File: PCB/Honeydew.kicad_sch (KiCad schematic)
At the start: 9 parts

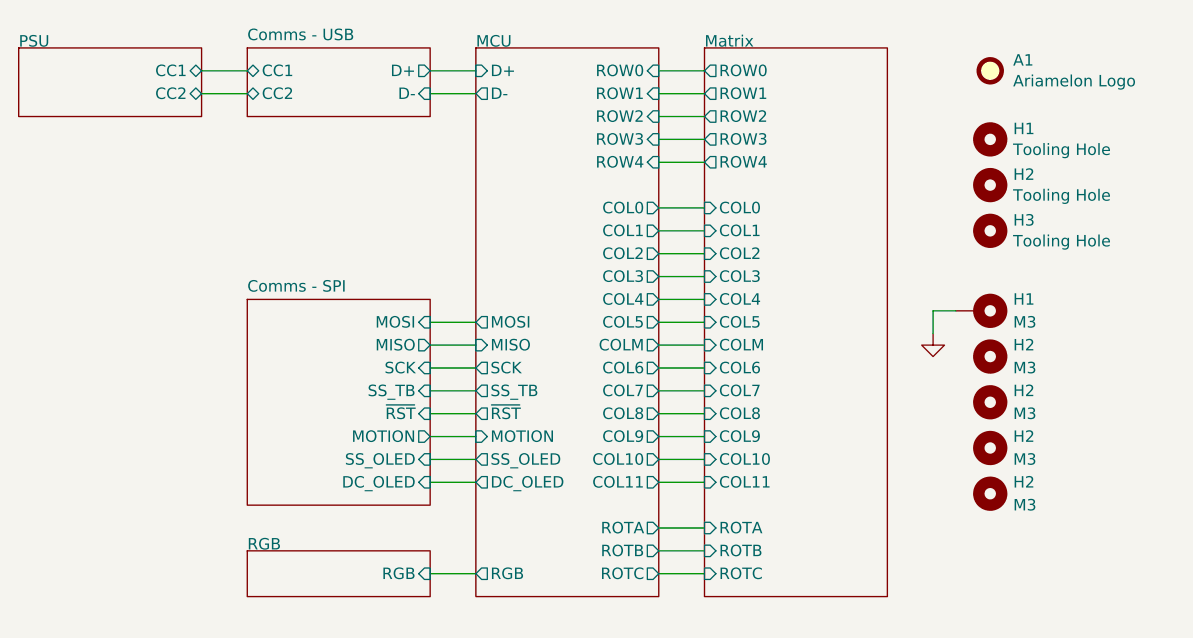
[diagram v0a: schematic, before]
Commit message: 17/04/2023 large update.
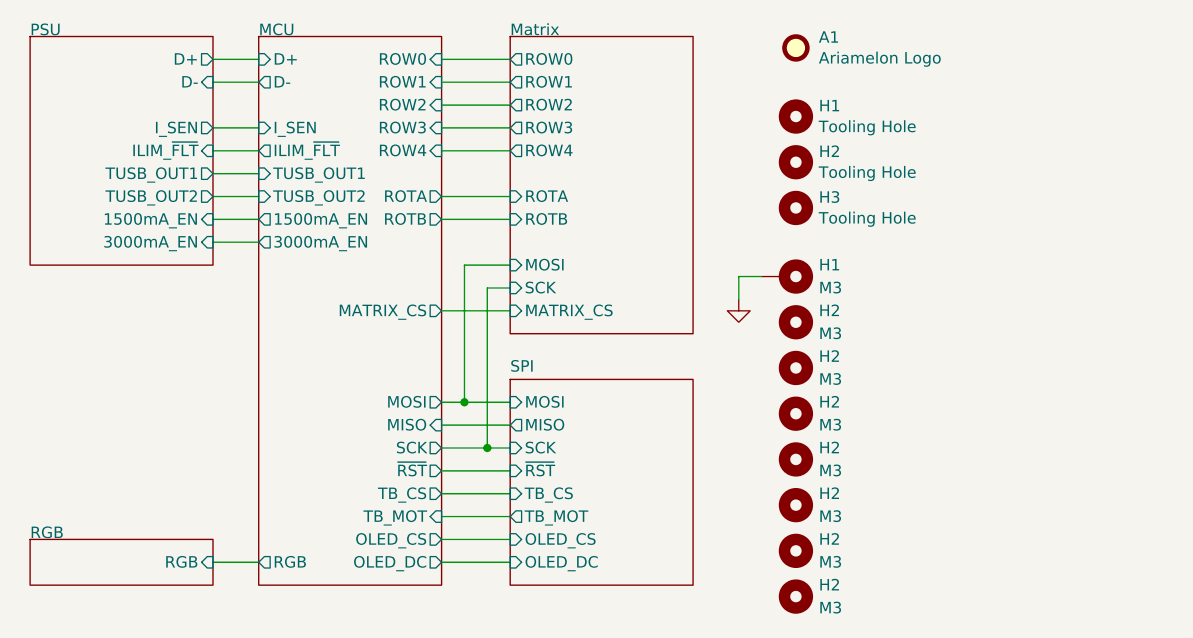
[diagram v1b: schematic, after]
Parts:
- added H2 (x3): M3, Honeydew:MountingHole_3.2mm_M3_Pad, symbol Mechanical:MountingHole
- A1: footprint Honeydew:Ariamelon_Logo_x3_CU -> Honeydew:Ariamelon_Logo_x3
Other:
- sheet Comms - SPI renamed SPI
- removed sheet Comms - USB
- sheet MCU ports: added 1500mA_EN, 3000mA_EN, ILIM_~{FLT}, I_SEN, MATRIX_CS, OLED_CS, OLED_DC, TB_CS, TB_MOT, TUSB_OUT1, TUSB_OUT2; removed COL0, COL1, COL10, COL11, COL2, COL3, COL4, COL5, COL6, COL7, COL8, COL9, COLM, DC_OLED, MOTION, ROTC, SS_OLED, SS_TB
- sheet Matrix ports: added MATRIX_CS, MOSI, SCK; removed COL0, COL1, COL10, COL11, COL2, COL3, COL4, COL5, COL6, COL7, COL8, COL9, COLM, ROTC
- sheet PSU ports: added 1500mA_EN, 3000mA_EN, D+, D-, ILIM_~{FLT}, I_SEN, TUSB_OUT1, TUSB_OUT2; removed CC1, CC2
- sheet SPI: file Comms - SPI.kicad_sch -> SPI.kicad_sch
- sheet SPI ports: added OLED_CS, OLED_DC, TB_CS, TB_MOT; removed DC_OLED, MOTION, SS_OLED, SS_TB
- moved on the sheet: A1, H1, H2, H3
